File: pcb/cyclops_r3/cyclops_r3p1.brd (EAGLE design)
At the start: 69.8 x 53.3 mm, 48 parts, among them Q1 SUM11006, Q2 IRF510, U1 MCP4921, U2 317-N, U3 ADR03, U4 OP1177, U5 LM324N, U6 ZXTD45

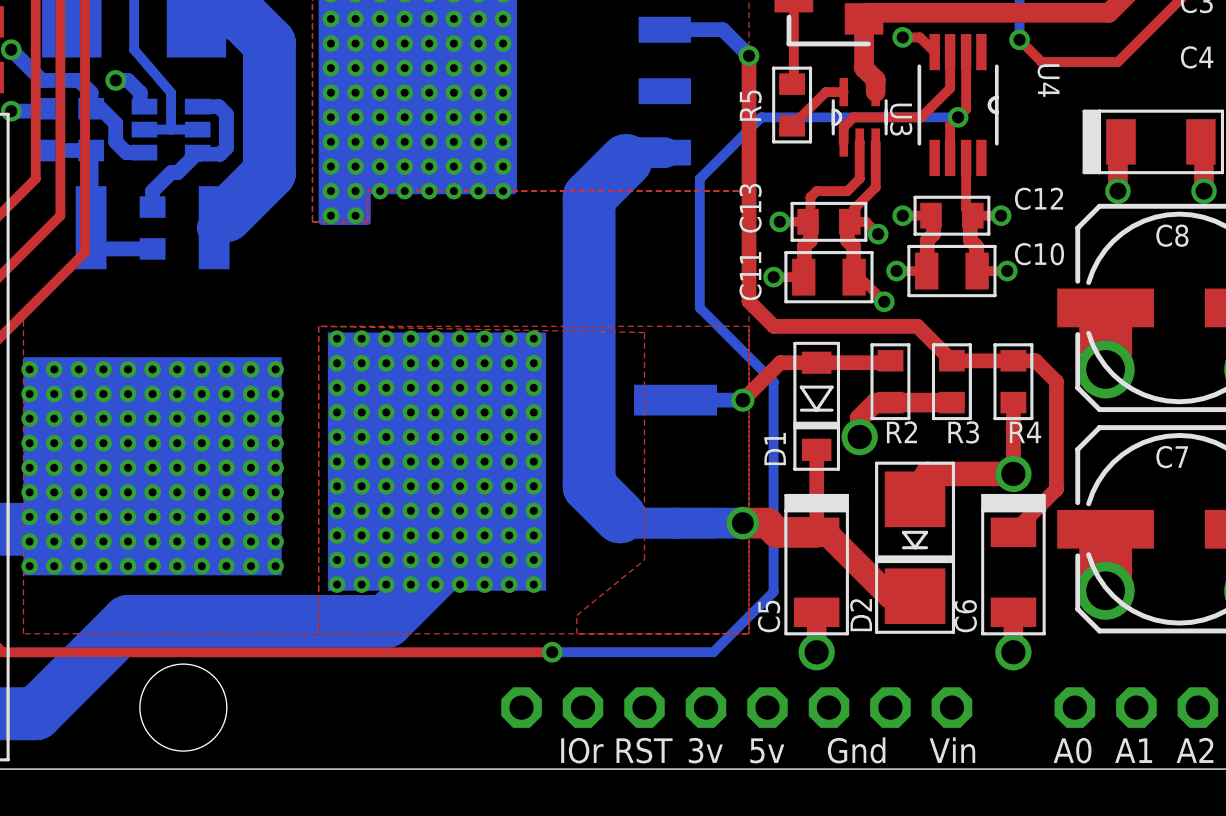
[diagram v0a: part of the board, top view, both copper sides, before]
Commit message: Minor changes.
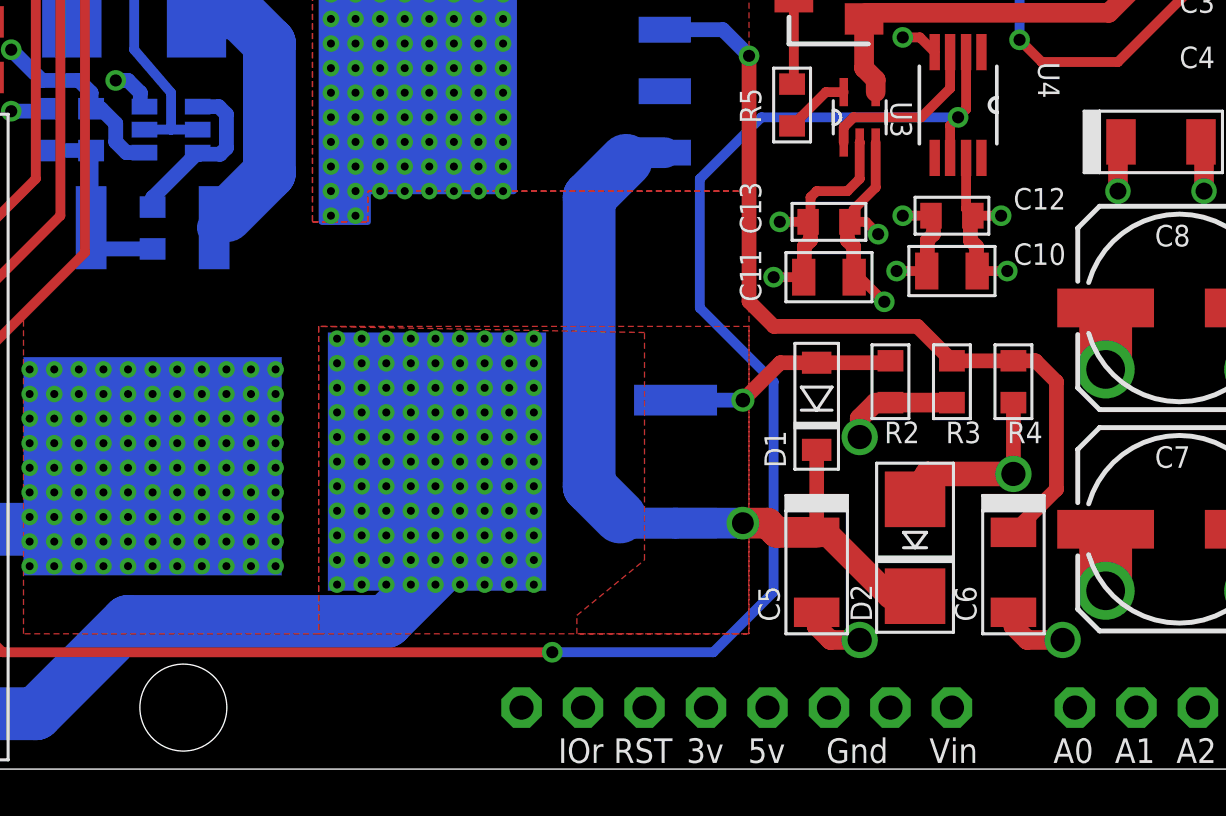
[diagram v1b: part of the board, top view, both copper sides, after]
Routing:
- net GND: track 65.8 -> 67.9 mm
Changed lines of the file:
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@@
 </plain>
 <attributes>
+<attribute name="PCB" value="Cyclops r3.1"/>
+<attribute name="REVISION" value="3.1"/>
 </attributes>
 <variantdefs>
@@
 </element>
 <element name="D2" library="cyclops" package="SMA-DO214AC" value="S1B" x="44.196" y="9.144" smashed="yes" rot="R270">
-<attribute name="NAME" x="42.418" y="5.588" size="0.889" layer="25" font="vector" ratio="18" rot="R90"/>
-<attribute name="VALUE" x="42.418" y="7.366" size="0.889" layer="27" font="vector" ratio="18" rot="R90"/>
+<attribute name="NAME" x="42.418" y="6.096" size="0.889" layer="25" font="vector" ratio="18" rot="R90"/>
+<attribute name="VALUE" x="42.418" y="8.128" size="0.889" layer="27" font="vector" ratio="18" rot="R90"/>
 </element>
 <element name="R3" library="cyclops" package="0603" value="1.8k" x="45.72" y="16.002" smashed="yes" rot="R90">
@@
 </element>
 <element name="C5" library="cyclops" package="1206-POL" value="1uF" x="40.132" y="8.128" smashed="yes" rot="R270">
-<attribute name="NAME" x="38.608" y="5.588" size="0.889" layer="25" font="vector" ratio="18" rot="R90"/>
-<attribute name="VALUE" x="38.608" y="7.62" size="0.889" layer="27" font="vector" ratio="18" rot="R90"/>
+<attribute name="NAME" x="38.608" y="6.096" size="0.889" layer="25" font="vector" ratio="18" rot="R90"/>
+<attribute name="VALUE" x="38.608" y="8.128" size="0.889" layer="27" font="vector" ratio="18" rot="R90"/>
 </element>
 <element name="C6" library="cyclops" package="1206-POL" value="10uF" x="48.26" y="8.128" smashed="yes" rot="R270">
-<attribute name="NAME" x="46.736" y="5.588" size="0.889" layer="25" font="vector" ratio="18" rot="R90"/>
-<attribute name="VALUE" x="46.736" y="7.62" size="0.889" layer="27" font="vector" ratio="18" rot="R90"/>
+<attribute name="NAME" x="46.736" y="6.096" size="0.889" layer="25" font="vector" ratio="18" rot="R90"/>
+<attribute name="VALUE" x="46.736" y="8.128" size="0.889" layer="27" font="vector" ratio="18" rot="R90"/>
 </element>
 <element name="C9" library="cyclops" package="1206-POL" value="1uF" x="54.356" y="25.908" smashed="yes">
@@
 <wire x1="58.168" y1="9.146" x2="58.168" y2="9.906" width="1.27" layer="1"/>
 <via x="41.91" y="13.716" extent="1-16" drill="1" shape="octagon"/>
-<via x="40.132" y="4.826" extent="1-16" drill="1" shape="octagon"/>
-<via x="48.26" y="4.826" extent="1-16" drill="1" shape="octagon"/>
-<wire x1="40.132" y1="4.826" x2="40.132" y2="6.477" width="0.8128" layer="1"/>
-<wire x1="48.26" y1="4.826" x2="48.26" y2="6.477" width="0.8128" layer="1"/>
+<via x="41.91" y="5.334" extent="1-16" drill="1" shape="octagon"/>
+<via x="50.292" y="5.334" extent="1-16" drill="1" shape="octagon"/>
+<wire x1="41.91" y1="5.334" x2="40.699959375" y2="5.334" width="0.8128" layer="1"/>
+<wire x1="40.699959375" y1="5.334" x2="40.132" y2="5.901959375" width="0.8128" layer="1"/>
+<wire x1="40.132" y1="5.901959375" x2="40.132" y2="6.477" width="0.8128" layer="1"/>
+<wire x1="50.292" y1="5.334" x2="48.827959375" y2="5.334" width="0.8128" layer="1"/>
+<wire x1="48.827959375" y1="5.334" x2="48.26" y2="5.901959375" width="0.8128" layer="1"/>
+<wire x1="48.26" y1="5.901959375" x2="48.26" y2="6.477" width="0.8128" layer="1"/>
 <wire x1="45.72" y1="15.1384" x2="43.18" y2="15.1384" width="0.8128" layer="1"/>
 <wire x1="43.18" y1="15.1384" x2="42.56055625" y2="15.1384" width="0.8128" layer="1"/>
@@
 <wire x1="15.494" y1="25.4" x2="14.628" y2="25.4" width="0.6096" layer="16"/>
 <wire x1="14.628" y1="25.4" x2="14.562" y2="25.466" width="0.6096" layer="16"/>
-<wire x1="12.7" y1="23.2156" x2="12.7" y2="23.876" width="0.6096" layer="16"/>
-<wire x1="12.7" y1="23.876" x2="13.462" y2="24.638" width="0.6096" layer="16"/>
-<wire x1="13.462" y1="24.638" x2="13.734" y2="24.638" width="0.6096" layer="16"/>
-<wire x1="13.734" y1="24.638" x2="14.562" y2="25.466" width="0.6096" layer="16"/>
+<wire x1="14.562" y1="25.466" x2="12.7" y2="23.604" width="0.6096" layer="16"/>
+<wire x1="12.7" y1="23.604" x2="12.7" y2="23.2156" width="0.6096" layer="16"/>
 </signal>
 <signal name="N$13">
